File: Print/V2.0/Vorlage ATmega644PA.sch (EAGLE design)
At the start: 59 parts, among them IC1 ATmega644PA, IC4 ATTINY24/44/84-SSU, Q1 16MHz, X2 87758-0616

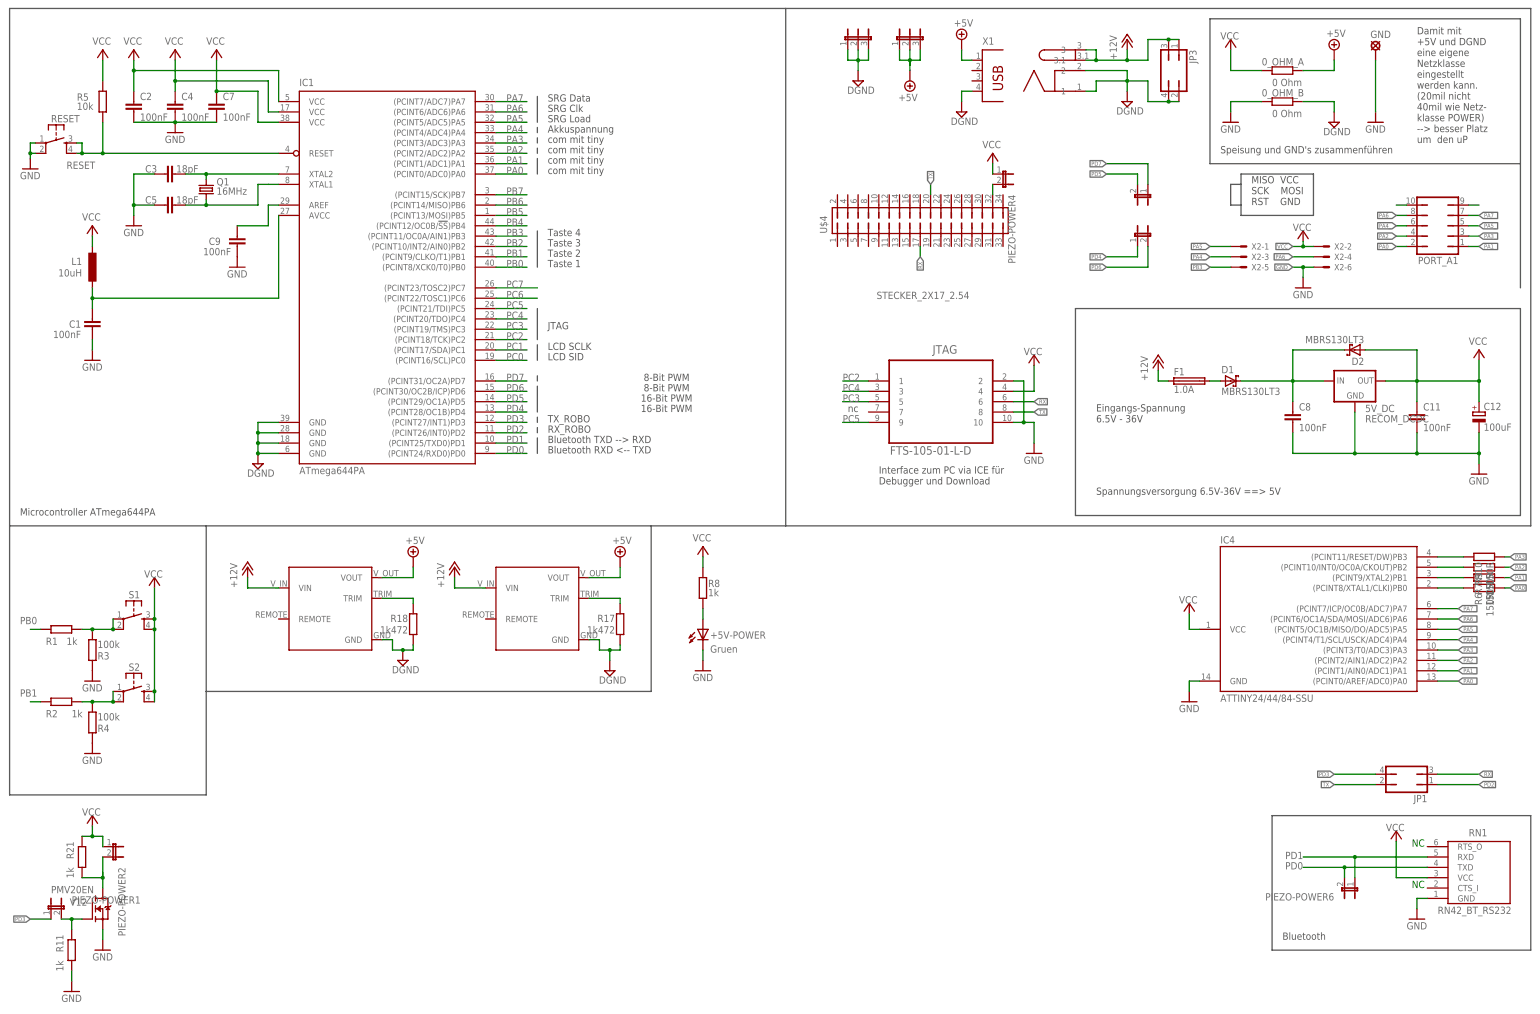
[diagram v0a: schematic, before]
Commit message: print fertig
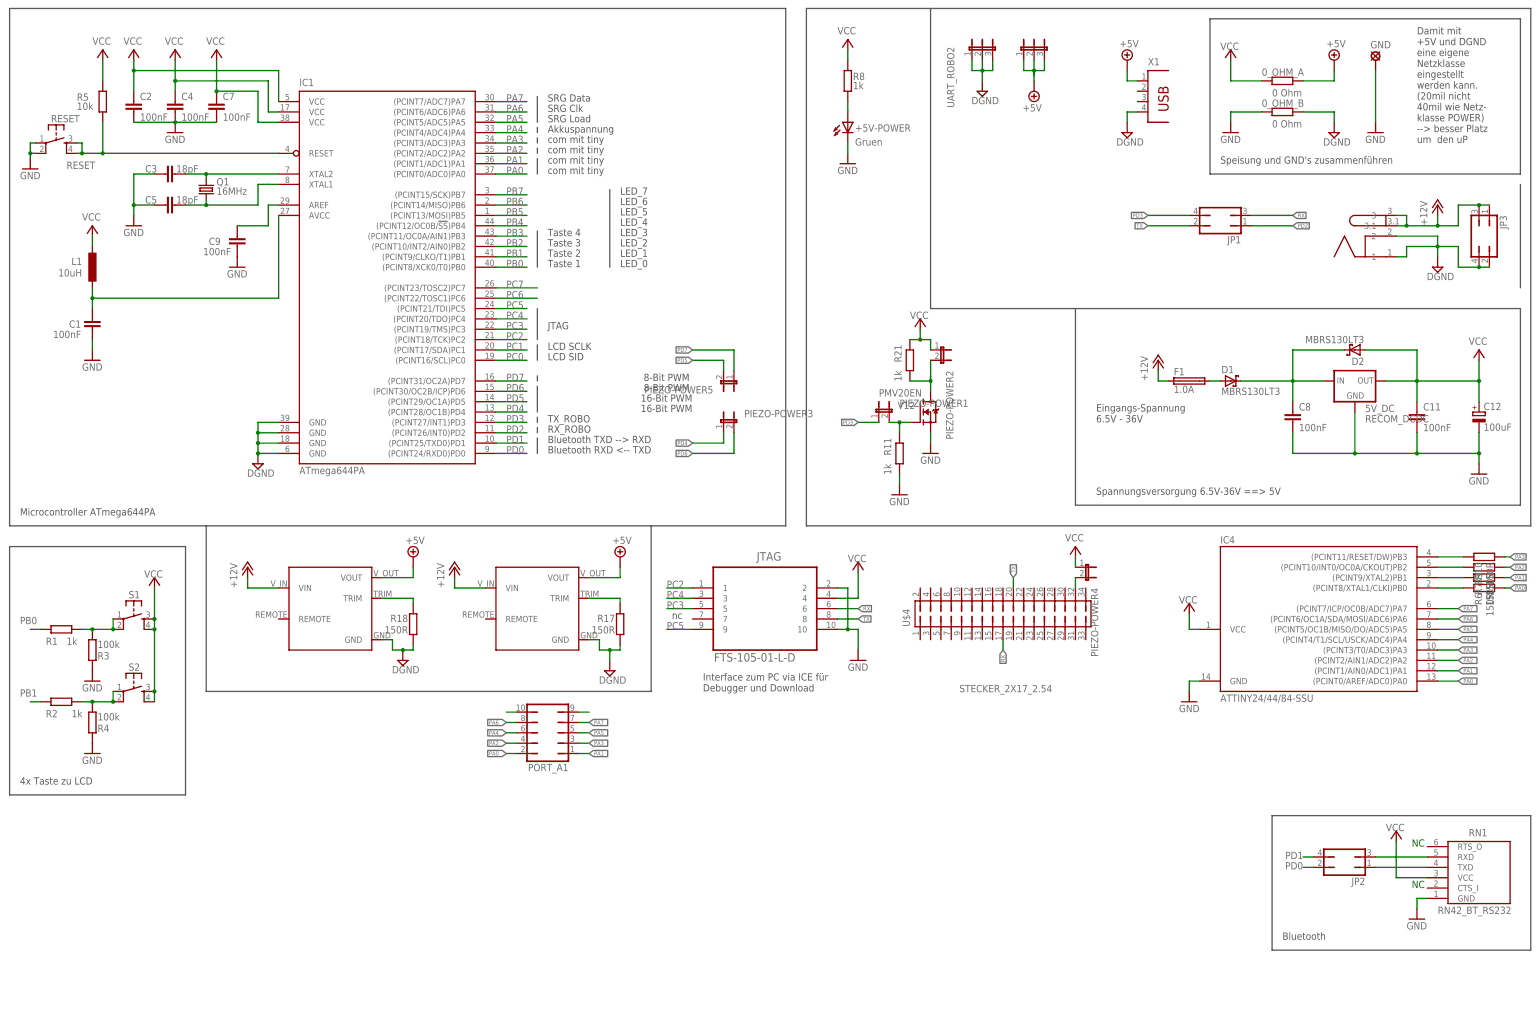
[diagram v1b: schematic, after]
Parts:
- removed PIEZO-POWER6: (no value), jumper:JP1E
- removed X2: 87758-0616, con-molex:87758-0616
- added JP2: (no value), jumper:JP2Q
- R17, R18: value 1k472 -> 150R
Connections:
- net PB0_ renamed N$7
- net PB1_ renamed N$6
- net PB2_ renamed N$5
- removed net PB3_: IC4.(PCINT11/RESET/DW)PB3, R10.2, X2-5.S
- new net N$14: JP2.3, RN1.RXD
- new net N$15: JP2.1, RN1.TXD
- new net N$3: IC4.(PCINT11/RESET/DW)PB3, R10.2
- net GND: no longer X2-6.S
- net PA4_: no longer X2-3.S
- net PA5_: no longer X2-1.S
- net PA6_: no longer X2-4.S
- net PD0: now also JP2.2; no longer PIEZO-POWER6.2, RN1.TXD
- net PD1: now also JP2.4; no longer PIEZO-POWER6.1, RN1.RXD
- net VCC: no longer X2-2.S
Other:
- note added: "4x Taste zu LCD"
- note added: "LED_0"
- note added: "LED_1"
- note added: "LED_2"
- note added: "LED_3"
- note added: "LED_4"
- note added: "LED_5"
- note added: "LED_6"
- note added: "LED_7"
- note removed: "MISO VCC SCK MOSI RST GND"
- moved on the sheet: +5V-POWER, 0_OHM_A, 0_OHM_B, GND, JP1, JP3, JTAG, PIEZO-POWER1, PIEZO-POWER2, PIEZO-POWER4, PORT_A1, R11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
